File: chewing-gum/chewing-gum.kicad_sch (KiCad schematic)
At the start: 19 parts, among them IC9 INA212AIDCKR, J15 Conn_02x01, J23 Conn_02x01, J28 Conn_01x03, J36 Conn_01x01_Socket, J42 Conn_Coaxial, J78 Conn_01x03, U21 TLV75801PDBV

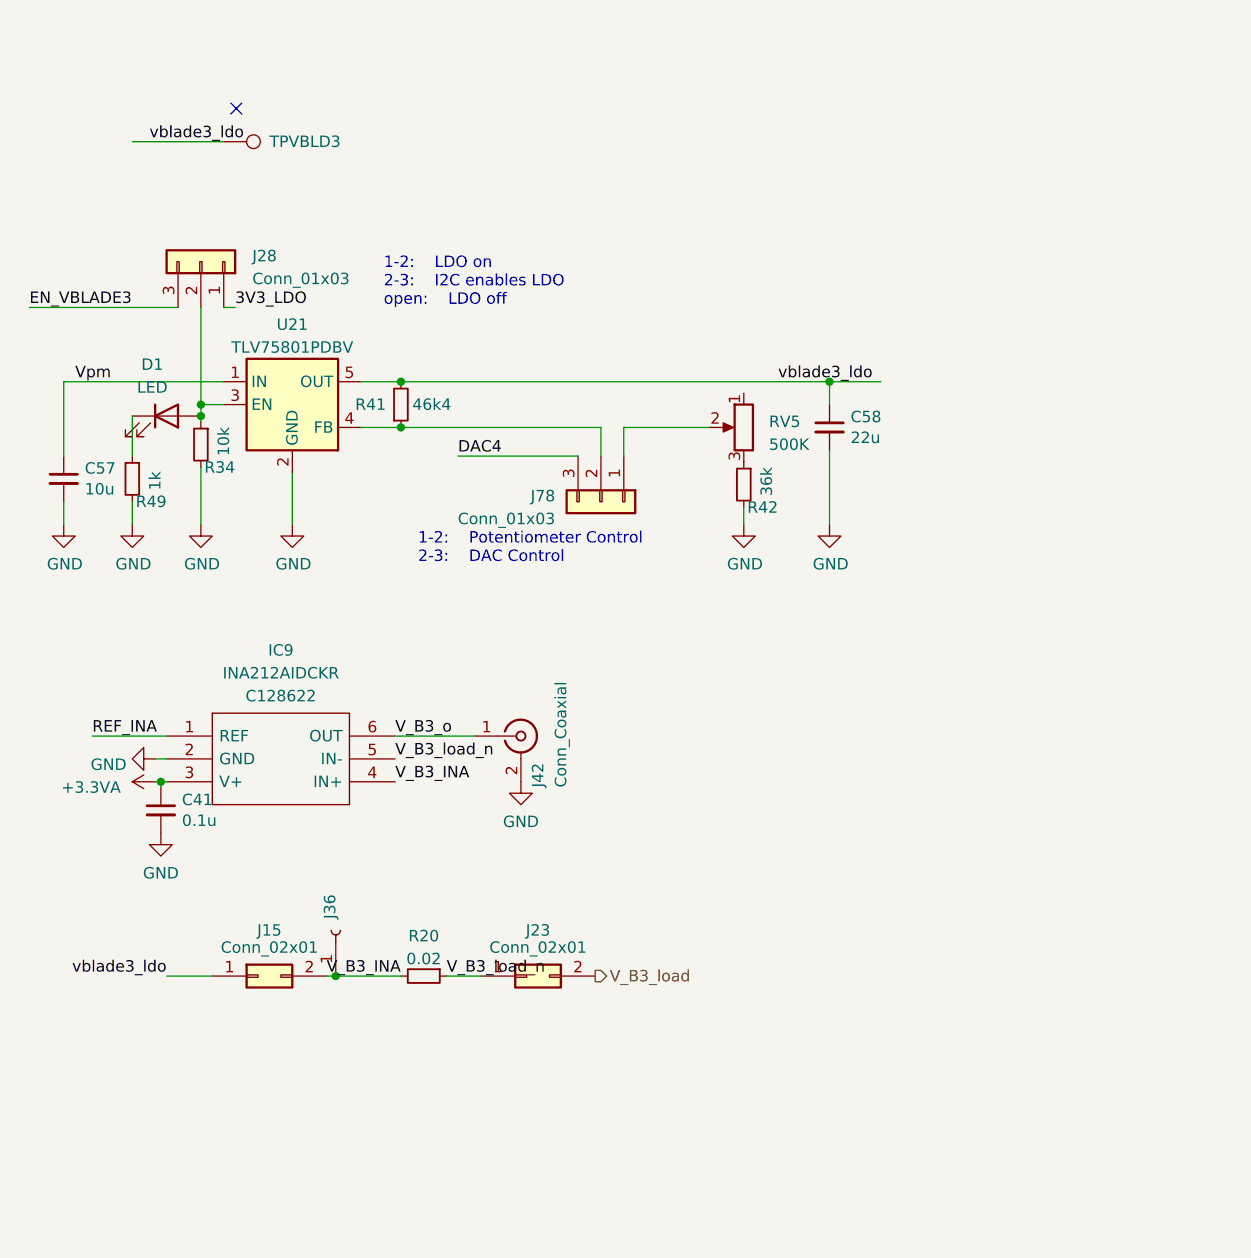
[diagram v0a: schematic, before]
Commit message: First version of the chewing gum Vdc
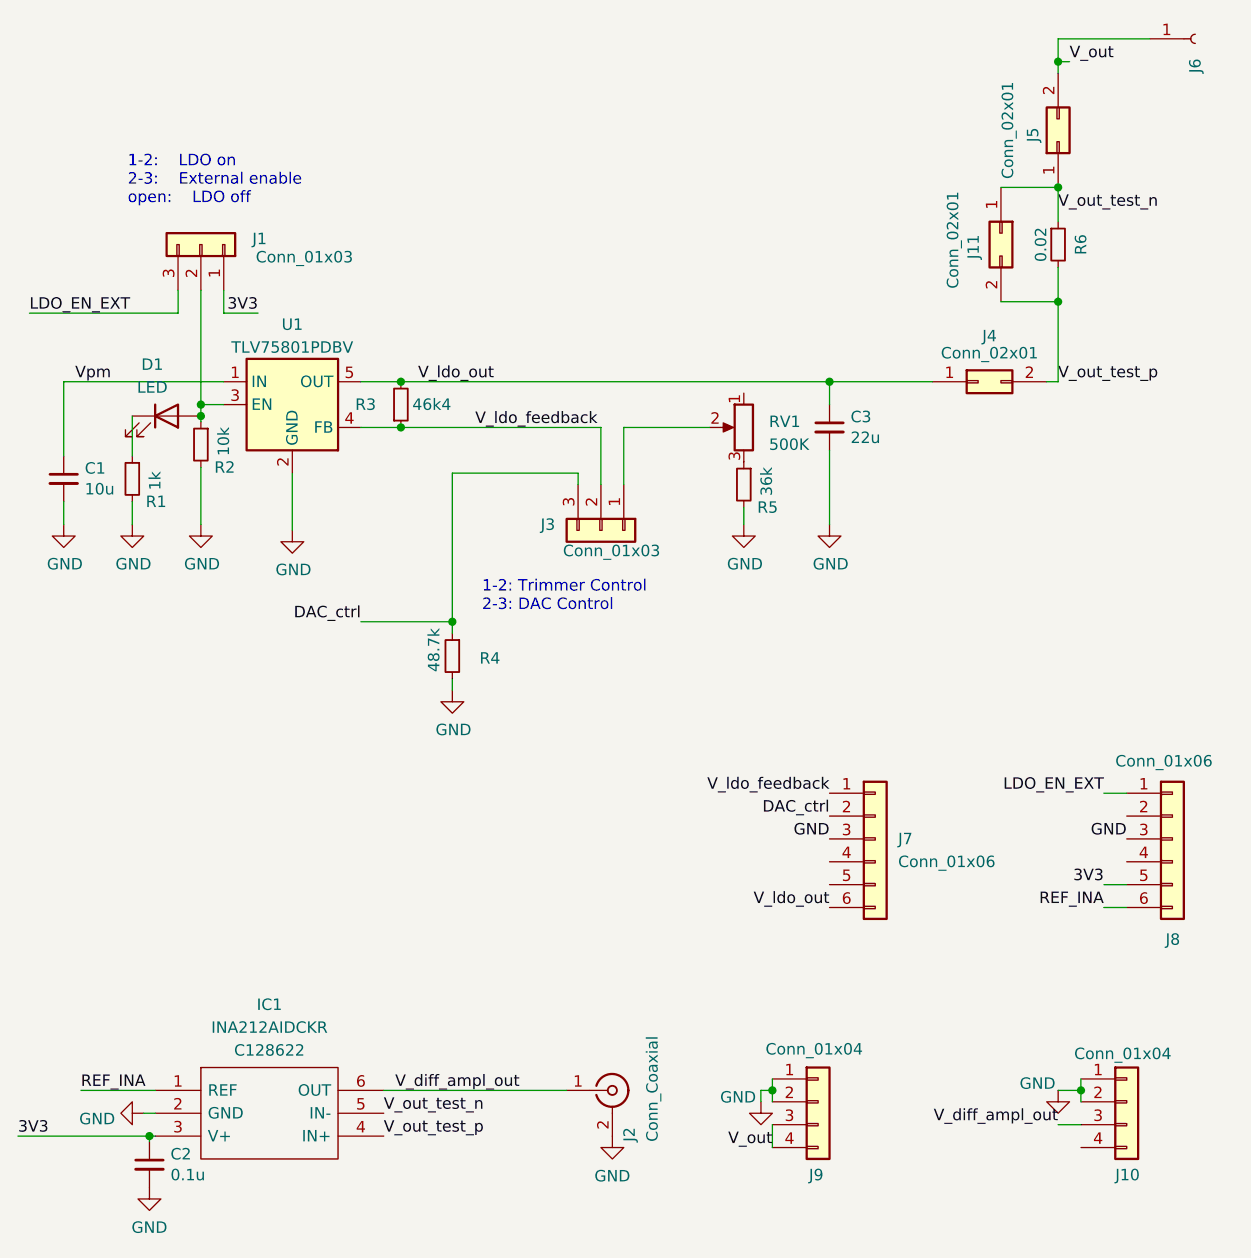
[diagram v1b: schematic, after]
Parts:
- removed J36: Conn_01x01_Socket, Connector:Banana_Jack_1Pin, symbol Connector:Conn_01x01_Socket
- removed TPVBLD3: TestPoint, TestPoint:TestPoint_Plated_Hole_D2.0mm, symbol Connector:TestPoint
- added J10, J9: Conn_01x04, Connector_PinHeader_1.27mm:PinHeader_1x04_P1.27mm_Vertical, symbol Connector_Generic:Conn_01x04
- added J11: Conn_02x01, Connector_PinHeader_2.54mm:PinHeader_1x02_P2.54mm_Vertical, symbol Connector_Generic:Conn_02x01
- added J6: Conn_01x01_Socket, Connector:Banana_Jack_1Pin, symbol Connector:Conn_01x01_Socket
- added J7, J8: Conn_01x06, Connector_PinHeader_1.27mm:PinHeader_1x06_P1.27mm_Vertical, symbol Connector_Generic:Conn_01x06
- added R4: 48.7k, Resistor_SMD:R_0603_1608Metric, symbol Device:R_Small
- renumbered C57 to C1, C41 to C2, C58 to C3, IC9 to IC1, J28 to J1, J42 to J2, J78 to J3, J15 to J4, J23 to J5, R49 to R1, R34 to R2, R41 to R3, R42 to R5, R20 to R6, RV5 to RV1, U21 to U1
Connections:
- net 3V3_LDO is gone; now on net 3V3: J1.1 (Pin_1)
- net GND: now also J10.1 (Pin_1), J10.2 (Pin_2), J7.3 (Pin_3), J8.3 (Pin_3), J9.1 (Pin_1), J9.2 (Pin_2), R4.2
- net REF_INA: now also J8.6 (Pin_6)
- net V_ldo_feedback: now reaches J3.2 (Pin_2), R3.1, U1.4 (FB)
- net V_ldo_feedback: now also J7.1 (Pin_1)
- net +3.3VA renamed 3V3
- net 3V3: now also J8.5 (Pin_5)
- net DAC4 renamed DAC_ctrl
- net DAC_ctrl: now also J7.2 (Pin_2), R4.1
- net EN_VBLADE3 renamed LDO_EN_EXT
- net LDO_EN_EXT: now also J8.1 (Pin_1)
- net V_B3_INA renamed V_out_test_p
- net V_out_test_p: now also J11.2 (Pin_2)
- net V_B3_load renamed V_out
- net V_out: now also J6.1 (Pin_1), J9.3 (Pin_3), J9.4 (Pin_4)
- net V_B3_load_n renamed V_out_test_n
- net V_out_test_n: now also J11.1 (Pin_1)
- net V_B3_o renamed V_diff_ampl_out
- net V_diff_ampl_out: now also J10.3 (Pin_3)
- net vblade3_ldo renamed V_ldo_out
- net V_ldo_out: now also J7.6 (Pin_6)
- no-connect marks 1 -> 0
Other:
- note added: "1-2: LDO on 2-3: External enable open: LDO off"
- note added: "1-2: Trimmer Control 2-3: DAC Control"
- note removed: "1-2: LDO on 2-3: I2C enables LDO open: LDO off"
- note removed: "1-2: Potentiometer Control 2-3: DAC Control"
- moved on the sheet: C2, IC1, J1, J2, J3, J4, J5, R6
